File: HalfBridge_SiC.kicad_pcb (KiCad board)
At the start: 2 copper layers, 100 x 100 mm, 56 parts, among them J1 Conn_02x08_Odd_Even, J2 AFBR-2624Z, J3 AFBR-2624Z, J4 Screw_Terminal_01x02, Q1 C3M0075120J, Q2 C3M0075120J, SW1 CAS-D20X1, U1 RKD-052005D, U2 RKD-052005D, U4 NCD57252

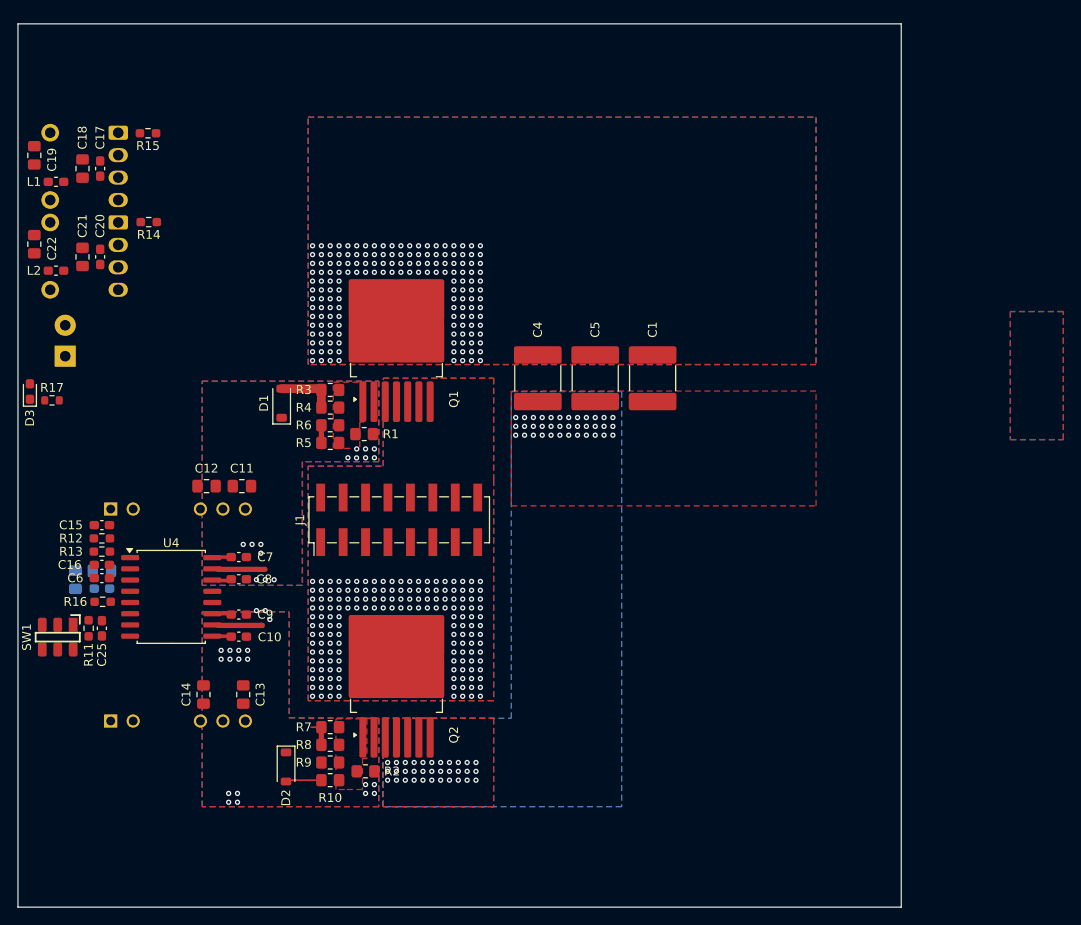
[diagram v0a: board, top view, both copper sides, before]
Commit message: diff rx
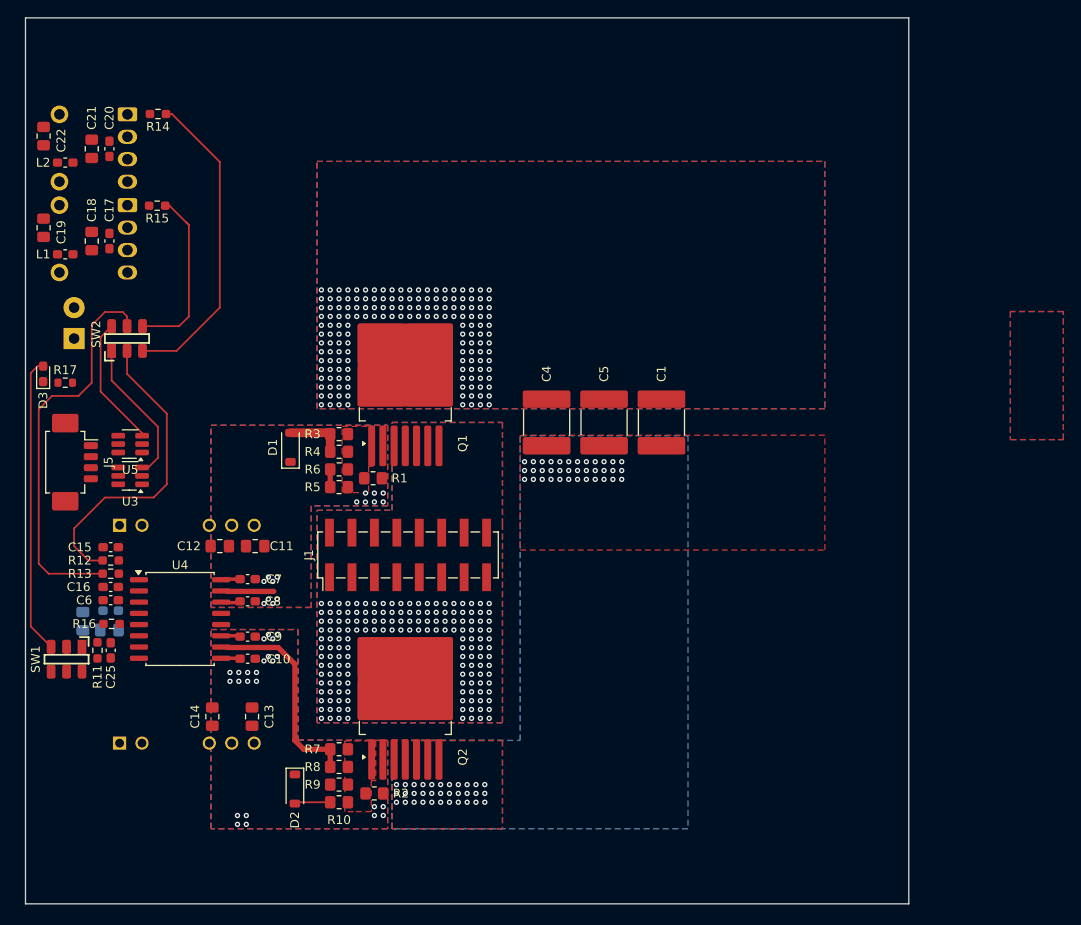
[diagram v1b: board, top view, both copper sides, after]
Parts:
- added J5: Conn_01x04, Connector_Molex:Molex_PicoBlade_53261-0471_1x04-1MP_P1.25mm_Horizontal, F.Cu at (45.0, 91.0)
- added SW2: CAS-D20X1, My_Button_Switch_SMD:Nidec_Copal_CAS-D20A1, F.Cu at (51.5, 77.0)
- added U3: MAX3284E, Package_TO_SOT_SMD:SOT-23-6_Handsoldering, F.Cu at (51.9, 92.5)
- added U5: MAX3284E, Package_TO_SOT_SMD:SOT-23-6_Handsoldering, F.Cu at (51.9, 89.0)
- moved C20 12.3 mm to (49.5, 55.5)
- moved C21 12.3 mm to (47.5, 55.5)
- moved J3 12.3 mm to (51.5, 51.6)
- moved R14 12.3 mm to (55.0, 51.6)
- moved C22 12.3 mm to (42.0, 54.1)
- moved L2 12.3 mm to (44.5, 57.1)
- moved C17 8.27 mm to (49.5, 66.0)
- moved C18 8.27 mm to (47.5, 66.0)
- moved C19 8.27 mm to (42.0, 64.5)
- moved L1 8.27 mm to (44.5, 67.5)
- moved J2 8.27 mm to (51.5, 61.9)
- moved R15 8.27 mm to (54.9, 62.0)
- moved C11 6.95 mm to (66.0, 100.5)
- moved C12 6.95 mm to (62.0, 100.5)
- moved C24 6.75 mm to (49.5, 110.0)
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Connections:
- net /HalfBridge_GateDriver/gnd renamed /HalfBridge_Diff/gnd
- net /HalfBridge_GateDriver/vcc renamed /HalfBridge_Diff/vcc
- C17 pad 1: /HalfBridge_Optical/vcca -> /HalfBridge_Optical/vccb
- C18 pad 1: /HalfBridge_Optical/vcca -> /HalfBridge_Optical/vccb
- C20 pad 1: /HalfBridge_Optical/vccb -> /HalfBridge_Optical/vcca
- C21 pad 1: /HalfBridge_Optical/vccb -> /HalfBridge_Optical/vcca
- J2 pad 1: /HalfBridge_Optical/xna -> /HalfBridge_Optical/xnb
- J2 pad 3: /HalfBridge_Optical/vcca -> /HalfBridge_Optical/vccb
- J3 pad 1: /HalfBridge_Optical/xnb -> /HalfBridge_Optical/xna
- J3 pad 3: /HalfBridge_Optical/vccb -> /HalfBridge_Optical/vcca
- L1 pad 1: /HalfBridge_Optical/vcca -> /HalfBridge_Optical/vccb
- L2 pad 1: /HalfBridge_Optical/vccb -> /HalfBridge_Optical/vcca
- R14 pad 1: /HalfBridge_GateDriver/inb -> /HalfBridge_Optical/ina
- R14 pad 2: /HalfBridge_Optical/xnb -> /HalfBridge_Optical/xna
- R15 pad 1: /HalfBridge_GateDriver/ina -> /HalfBridge_Optical/inb
- R15 pad 2: /HalfBridge_Optical/xna -> /HalfBridge_Optical/xnb
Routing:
- net /HalfBridge_GateDriver/inb: track 0.00 -> 44.9 mm
- net /HalfBridge_Optical/ina: track 0.00 -> 35.6 mm
- net /HalfBridge_GateDriver/ina: track 0.00 -> 35.4 mm
- net /HalfBridge_Diff/vcc: track 0.00 -> 33.7 mm
- net /HalfBridge_Optical/inb: track 0.00 -> 20.2 mm
- net /HalfBridge_Diff/ina_d: track 0.00 -> 17.0 mm
- net /HalfBridge_GateDriver/gonl: track 8.26 -> 24.8 mm
- net /HalfBridge_Diff/inb_d: track 0.00 -> 15.4 mm
- net /HalfBridge_GateDriver/kl: vias 19 -> 24
- net /HalfBridge_GateDriver/kh: vias 14 -> 15
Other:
- board size 100 x 100 mm -> 100 x 100.3 mm
- board text added: "INA PWM"
- board text removed: "INA"
